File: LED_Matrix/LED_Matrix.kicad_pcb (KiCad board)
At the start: 2 copper layers, 44.5 x 29.2 mm, 21 parts, among them J1 Conn_01x02, U1 NE555P

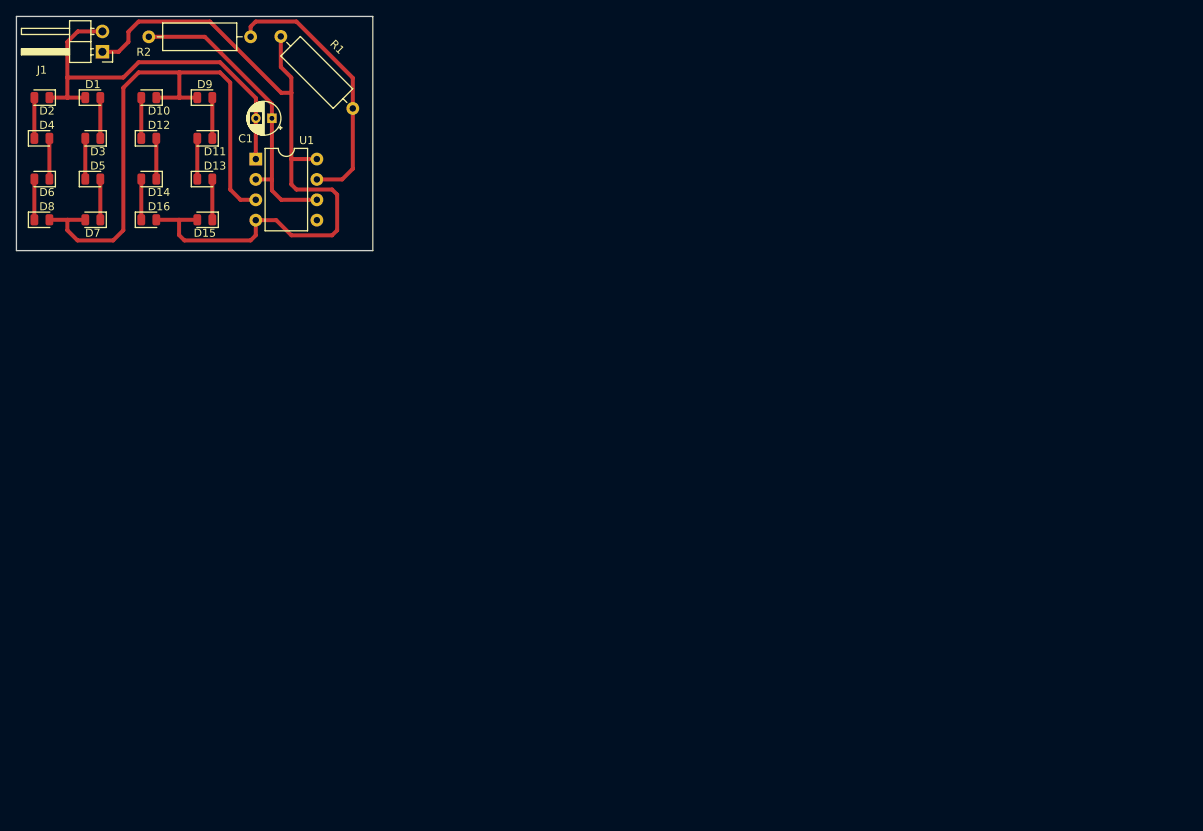
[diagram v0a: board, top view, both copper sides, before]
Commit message: 20230318_174200
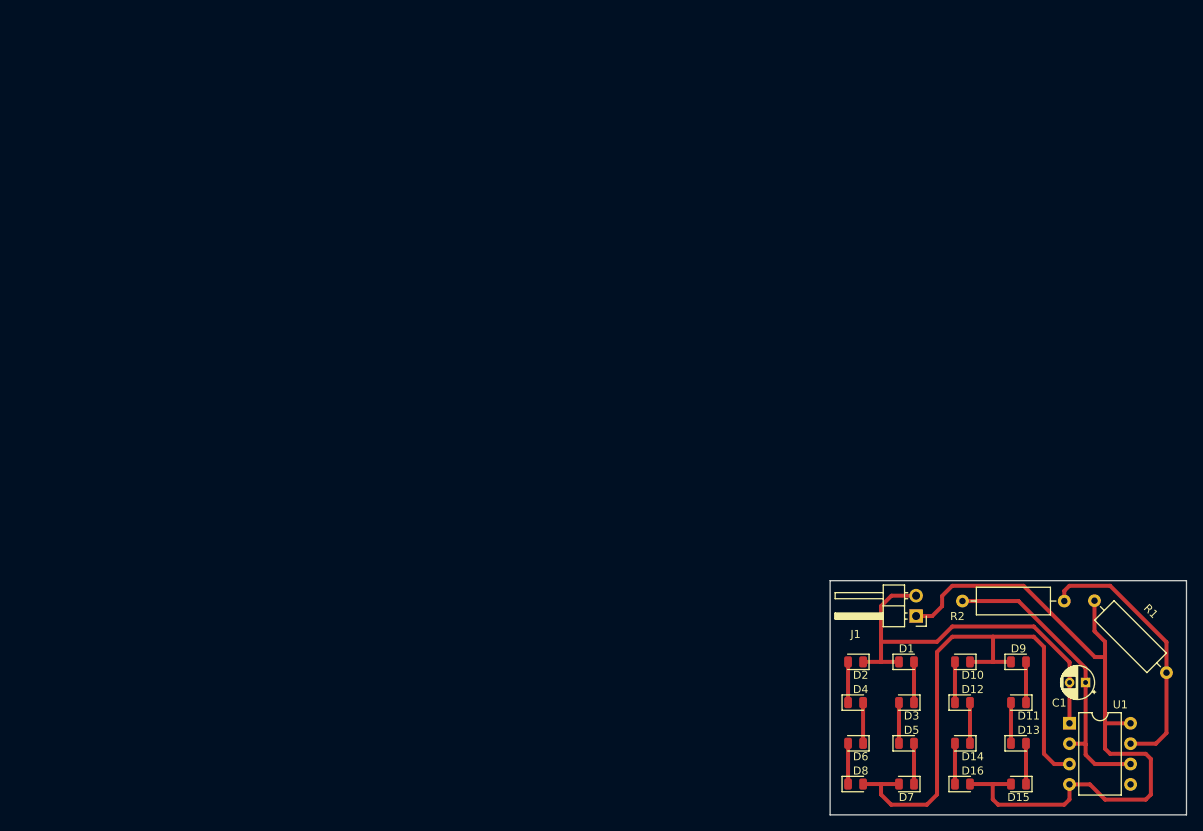
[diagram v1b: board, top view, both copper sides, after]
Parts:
- moved D16 123.5 mm to (139.6, 114.1)
- moved D8 123.5 mm to (126.2, 114.1)
- moved D1 123.5 mm to (132.6, 98.9)
- moved D11 123.5 mm to (146.6, 104.0)
- moved D13 123.5 mm to (146.6, 109.1)
- moved D15 123.5 mm to (146.6, 114.1)
- moved D3 123.5 mm to (132.6, 104.0)
- moved D5 123.5 mm to (132.6, 109.1)
- moved D7 123.5 mm to (132.6, 114.1)
- moved D9 123.5 mm to (146.6, 98.9)
- moved R1 123.5 mm to (156.0, 91.3)
- moved C1 123.5 mm to (154.9, 101.5)
- moved D10 123.5 mm to (139.6, 98.9)
- moved D12 123.5 mm to (139.6, 104.0)
- moved D14 123.5 mm to (139.6, 109.1)
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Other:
- board text added: "0"
- board text added: "0 mm"
- board text added: "0,01 mm"
- board text added: "0,02"
- board text added: "0,035 mm"
- board text added: "0,3000 mm"
- board text added: "0,5000 mm / 0,0000 mm"
- board text added: "1"
- board text added: "1,51 mm"
- board text added: "1,6000 mm"
- board text added: "2"
- board text added: "3,3"
- board text added: "4,5"
- board text added: "44,4500 mm x 29,2100 mm"
- board text added: "B.Cu"
- board text added: "B.Mask"
- board text added: "B.Paste"
- board text added: "B.Silkscreen"
- board text added: "Bottom Silk Screen"
- board text added: "Bottom Solder Mask"
- board text added: "Bottom Solder Paste"
- board text added: "F.Cu"
- board text added: "F.Mask"
- board text added: "F.Paste"
- board text added: "F.Silkscreen"
- board text added: "FR4"
- board text added: "None"
- board text added: "Not specified"
- board text added: "Top Silk Screen"
- board text added: "Top Solder Mask"
- board text added: "Top Solder Paste"
- board text added: "copper"
- board text added: "core"
- board text added: "Габариты платы:"
- board text added: "Диэлектрик"
- board text added: "Имя слоя"
- board text added: "Количество слоёв меди:"
- board text added: "Контроль импеданса:"
- board text added: "Краевой соединитель:"
- board text added: "Материал"
- board text added: "Метал. торцы:"
- board text added: "Мин. дорожка/зазор:"
- board text added: "Мин. сверло:"
- board text added: "Нет"
- board text added: "Отн.диэл.прон."
- board text added: "Периферийные полу-отверстия:"
- board text added: "Покрытие меди:"
- board text added: "Танг.угла диэл.потерь"
- board text added: "Тип"
- board text added: "Толщина (мм)"
- board text added: "Толщина платы:"
- board text added: "ХАРАКТЕРИСТИКИ ПЛАТЫ"
- board text added: "Цвет"
